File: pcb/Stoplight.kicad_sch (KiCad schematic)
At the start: 13 parts, among them IC1 ATtiny85-20M, IC2 AP7375-50SA-7, J1 Conn_ARM_SWD_TagConnect_TC203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

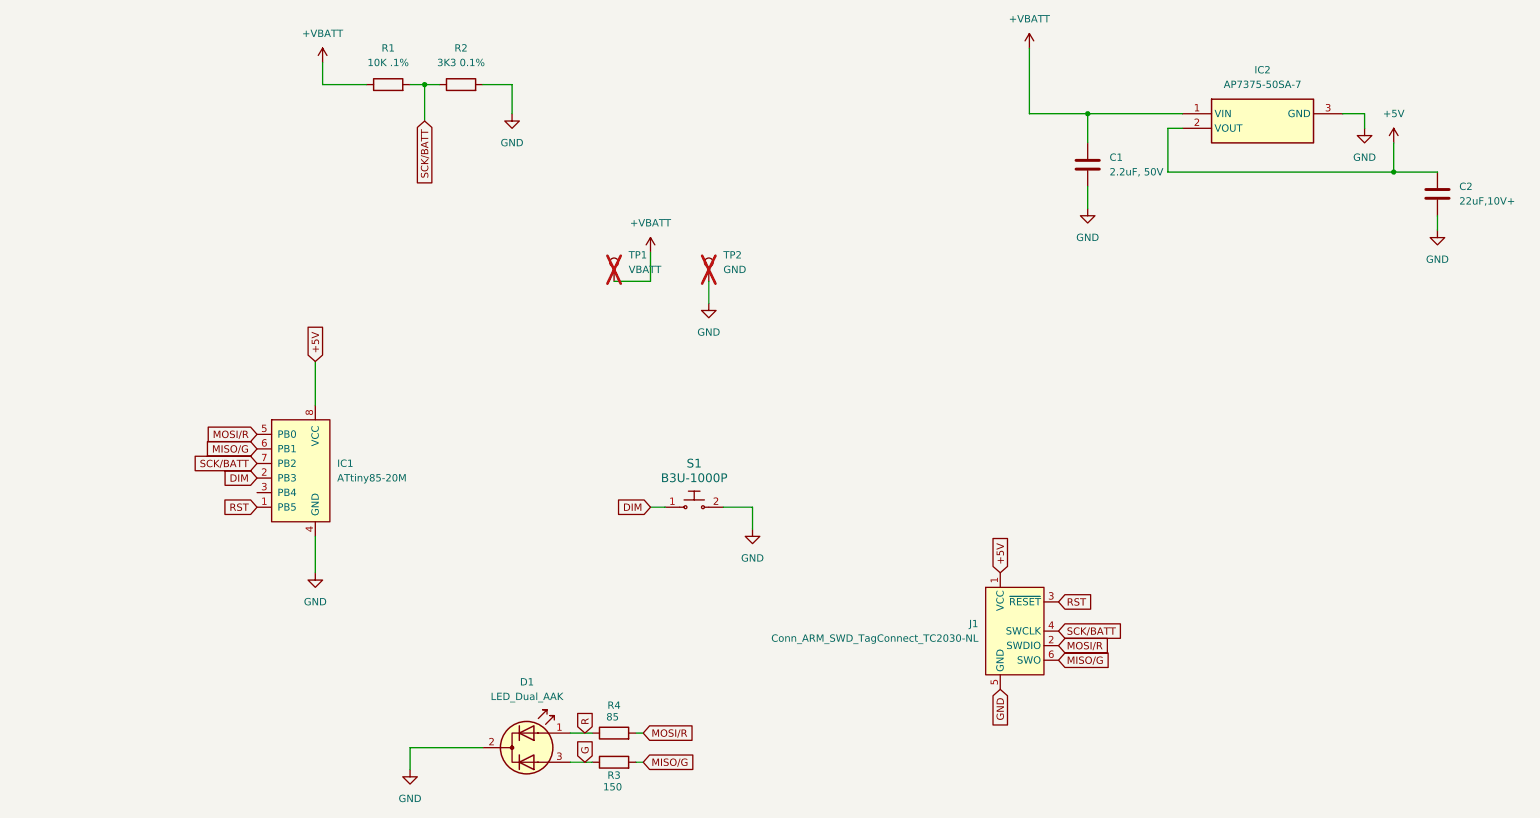
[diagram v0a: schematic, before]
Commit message: v1b PCB as ordered
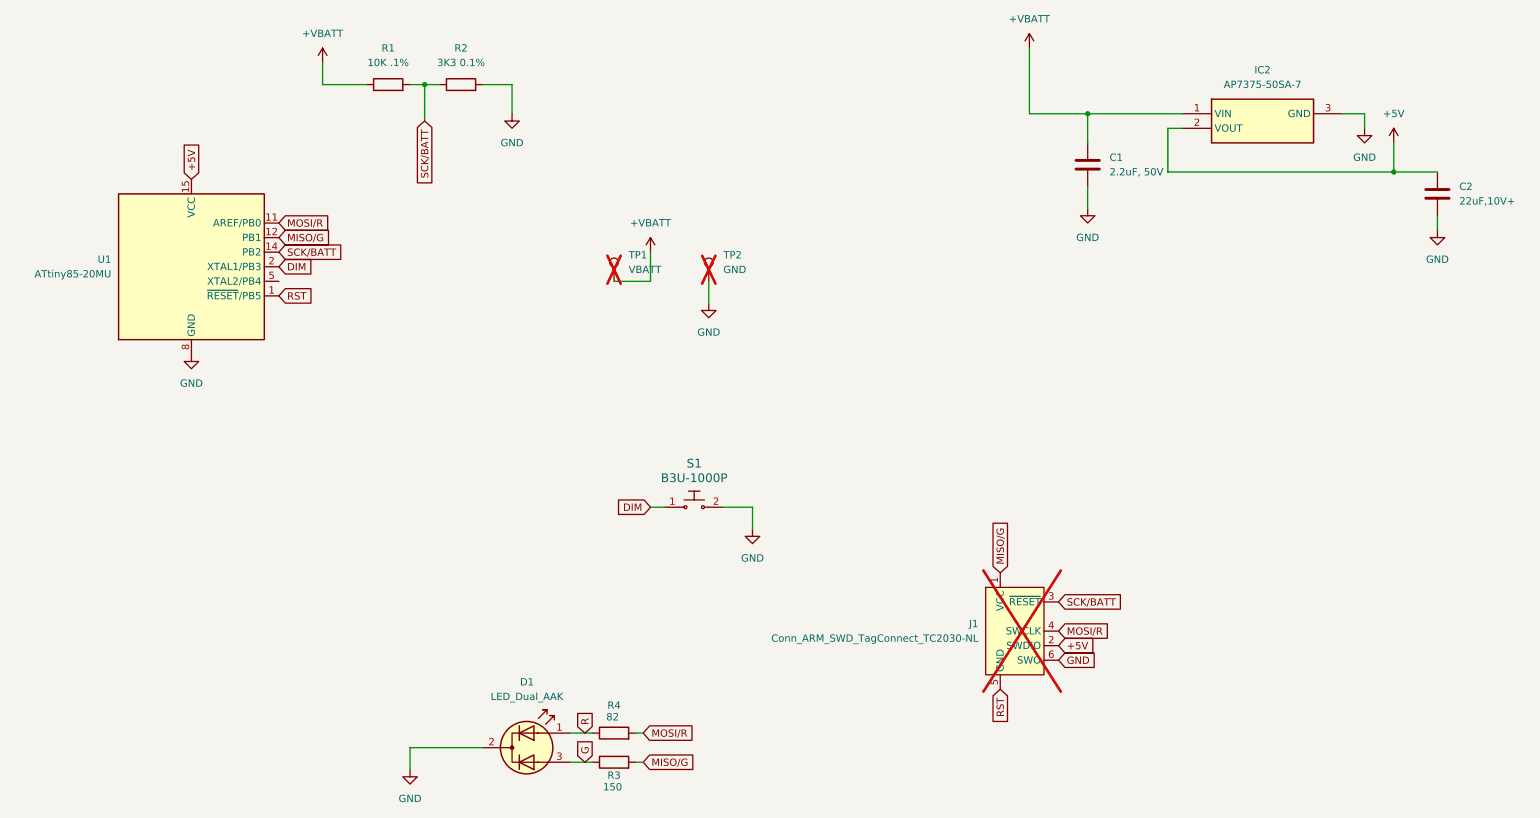
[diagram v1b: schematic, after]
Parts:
- removed IC1: ATtiny85-20M, digikey-footprints:SOIC-8_W3.9mm, symbol dk_Embedded-Microcontrollers:ATTINY85-20SU
- added U1: ATtiny85-20MU, Package_DFN_QFN:QFN-20-1EP_4x4mm_P0.5mm_EP2.6x2.6mm, symbol MCU_Microchip_ATtiny:ATtiny85-20M
- C1: footprint Capacitor_SMD:C_0805_2012Metric -> Capacitor_SMD:C_0603_1608Metric; Part Number C2012X7R2A225K125AC -> GRM188R61H225KE11D; URL https://www.digikey.com/en/products/detail/taiyo-yuden/UMK2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 -> https://www.digikey.com/en/products/detail/murata-electroni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
- C2: footprint Capacitor_SMD:C_0805_2012Metric -> Capacitor_SMD:C_0402_1005Metric
- J1: now not fitted; now in the parts list
- R1: footprint Resistor_SMD:R_0805_2012Metric -> Resistor_SMD:R_0402_1005Metric; Part Number ERA-1AEB103C -> 4-2176755-8; URL https://www.digikey.com/en/products/detail/panasonic-electr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 -> https://www.digikey.com/en/products/detail/te-connectivity-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
- R2: footprint Resistor_SMD:R_0805_2012Metric -> Resistor_SMD:R_0402_1005Metric; Part Number ERA-1AEB332C -> TNPW04023K30BEED; URL https://www.digikey.com/en/products/detail/panasonic-electr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 -> https://www.digikey.com/en/products/detail/vishay-dale/TNPW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
- R3: footprint Resistor_SMD:R_0805_2012Metric -> Resistor_SMD:R_0402_1005Metric; Part Number ERA-3AEB151V -> ERJ-PA2F1500X; URL https://www.digikey.com/en/products/detail/panasonic-electronic-components/ERA-3AEB151V/1465834 -> https://www.digikey.com/en/products/detail/panasonic-electronic-components/ERJ-PA2F1500X/5402645
- R4: value 85 -> 82; footprint Resistor_SMD:R_0805_2012Metric -> Resistor_SMD:R_0402_1005Metric; Part Number ERJ-3EKF84R5V -> ERJ-PA2F82R0X; URL https://www.digikey.com/en/products/detail/panasonic-electronic-components/ERJ-3EKF84R5V/196495 -> https://www.digikey.com/en/products/detail/panasonic-electronic-components/ERJ-PA2F82R0X/9815376?s=N4IgjCBcoExaBjKAzAhgGwM4FMA0IB7KAbXADYBWAFgGYQBdfABwBcoQBlFgJwEsA7AOYgAvvjrQQSSGix5CJcGBoRGIVuy58ho-BXhSUGHPiKRSKsgE4YADgbM2kTjwHCx5A9NkmF5kDRWYBT2ahrOWm664ADsXkZyporKMaGOmq46HlRk8TLG8makZCoADA7qTi7a7vhgMVR5PoWKVGD1VHBhVZFZ%2BDAUcJLeBUn%2BMJ1WNI3dGTXRMaVxwwm%2BReAV4dVRHu0wy4irLeObVQByAK4Atth8SLswQU2jfhZBFHGzEZm14BSl5RW%2BUSrxAVCCM3S33muwoKmeIPWqih2z64CstisCLWinK9A8MFKtn0QOaY1IthgAAIAPIACyumFO7AAqvxeCwacgALLYVCYC7cbDRAC0EFJLyReI8IsaEsRilstgadHx%2BBFJMOwJx-gg-RA-VoDBlB0M2uOxTAAIoFFwVuNIhEQA
- S1: Category Switches -> (none); DK_Datasheet_Link https://omronfs.omron.com/en_US/ecb/products/pdf/en-b3u.pdf -> (none); DK_Detail_Page /product-detail/en/omron-electronics-inc-emc-div/B3U-1000P/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 -> (none); Family Tactile Switches -> (none); MPN B3U-1000P -> (none); Manufacturer Omron Electronics Inc-EMC Div -> (none); Part Number (none) -> B3U-1000P; Status Active -> (none); URL (none) -> https://www.digikey.com/en/products/detail/omron-electronic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
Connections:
- net +5V: now also J1.2 (SWDIO), U1.15 (VCC); no longer J1.1 (VCC)
- net DIM: now also U1.2 (XTAL1/PB3)
- net GND: now also J1.6 (SWO), U1.21 (GND), U1.8 (GND); no longer J1.5 (GND)
- net MISO/G: now also J1.1 (VCC), U1.12 (PB1); no longer J1.6 (SWO)
- net MOSI/R: now also J1.4 (SWCLK), U1.11 (AREF/PB0); no longer J1.2 (SWDIO)
- net RST: now also J1.5 (GND), U1.1 (~{RESET}/PB5); no longer J1.3 (~{RESET})
- net SCK/BATT: now also J1.3 (~{RESET}), U1.14 (PB2); no longer J1.4 (SWCLK)
